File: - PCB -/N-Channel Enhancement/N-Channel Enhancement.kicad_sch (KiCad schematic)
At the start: 9 parts, among them J1 Conn_01x02_Pin, J2 Conn_01x01_Pin, J3 Conn_01x04_Pin, J4 Conn_01x01_Pin, Q2 NMOS

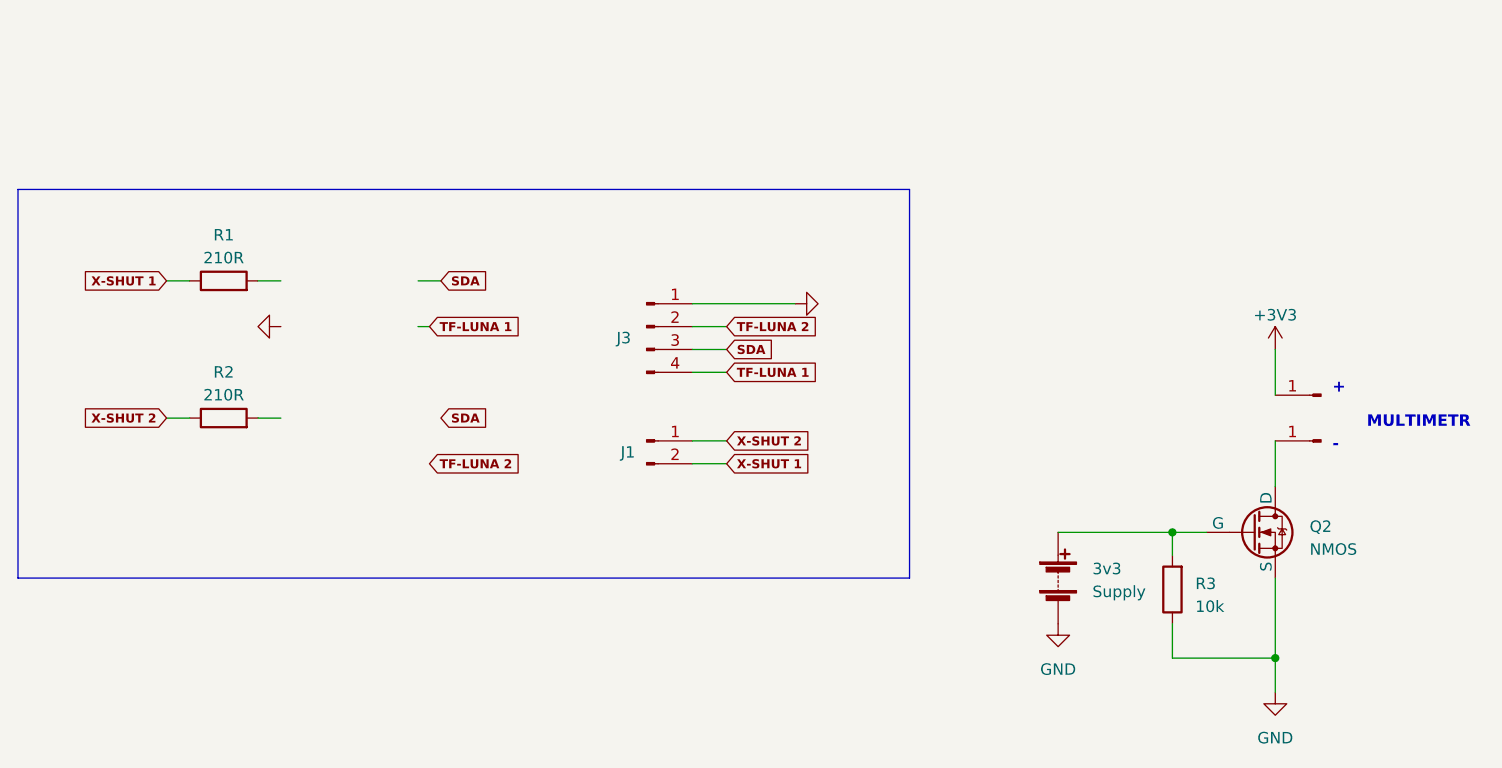
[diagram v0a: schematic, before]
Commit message: matej push
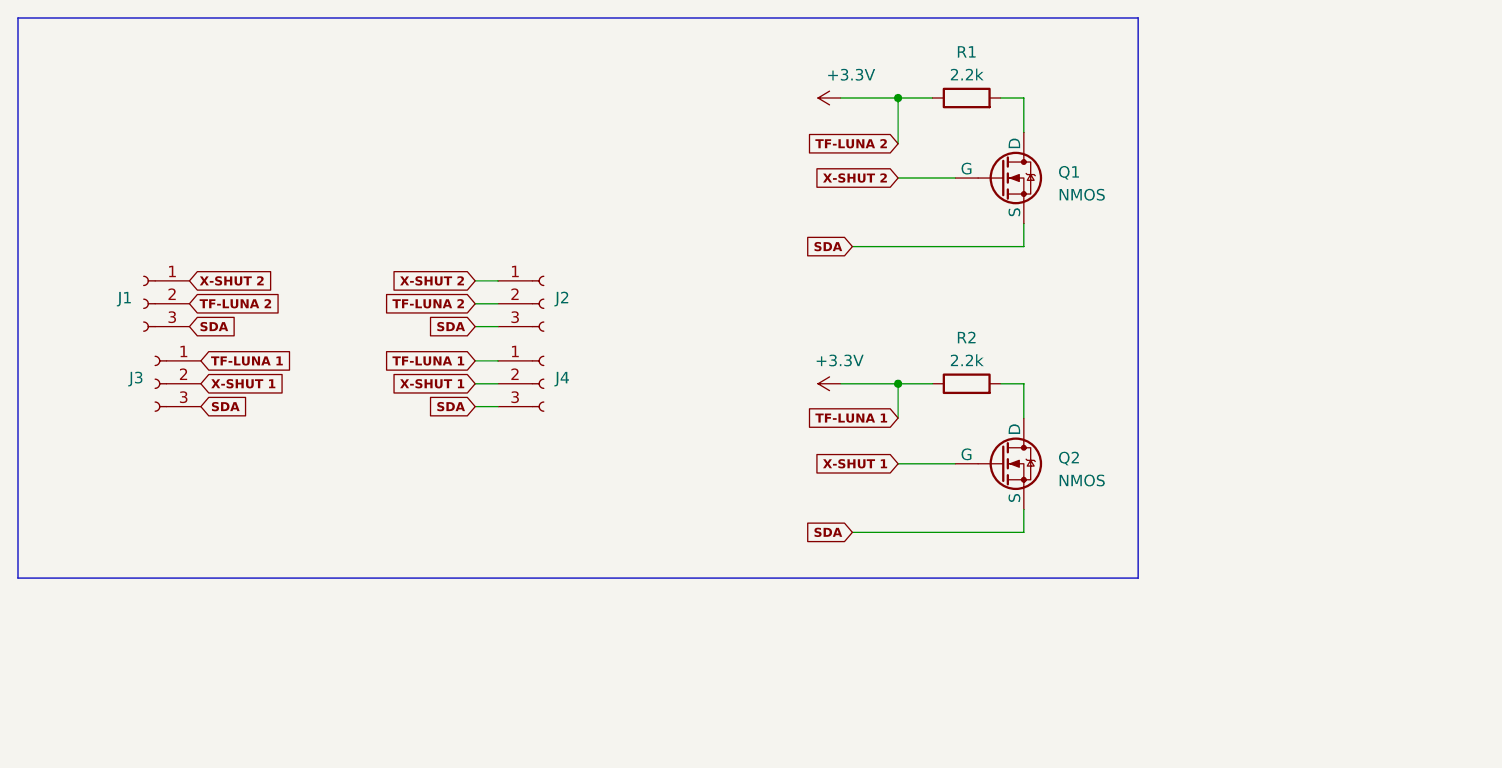
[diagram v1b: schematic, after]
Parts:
- removed 3v3: Supply, symbol Device:Battery
- removed J1: Conn_01x02_Pin, Connector_JST:JST_XH_B2B-XH-A_1x02_P2.50mm_Vertical, symbol Connector:Conn_01x02_Pin
- removed J2, J4: Conn_01x01_Pin, symbol Connector:Conn_01x01_Pin
- removed J3: Conn_01x04_Pin, Connector_JST:JST_XH_B4B-XH-A_1x04_P2.50mm_Vertical, symbol Connector:Conn_01x04_Pin
- removed R3: 10k, symbol Device:R
- added J1, J2, J3, J4: Conn_01x03_Socket, Connector_PinSocket_2.54mm:PinSocket_1x03_P2.54mm_Vertical, symbol Connector:Conn_01x03_Socket
- added Q1: NMOS, Package_TO_SOT_SMD:SOT-23, symbol Simulation_SPICE:NMOS
- Q2: footprint (none) -> Package_TO_SOT_SMD:SOT-23
- R1, R2: value 210R -> 2.2k
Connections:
- net GND is gone; now on net SDA: Q2.3 (S)
- net SDA: now also J1.3 (Pin_3), J2.3 (Pin_3), J3.3 (Pin_3), J4.3 (Pin_3), Q1.3 (S)
- net X-SHUT 1: now also Q2.2 (G), J3.2 (Pin_2), J4.2 (Pin_2); no longer R1.1
- net X-SHUT 2: now also J1.1 (Pin_1), J2.1 (Pin_1), Q1.2 (G); no longer R2.1
- net at Q2.1 (D): now also R2.2
- net at R1.2: now also Q1.1 (D)
- new net +3.3V: J1.2 (Pin_2), J2.2 (Pin_2), J3.1 (Pin_1), J4.1 (Pin_1), R1.1, R2.1
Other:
- note removed: "+"
- note removed: "-"
- note removed: "MULTIMETR"
